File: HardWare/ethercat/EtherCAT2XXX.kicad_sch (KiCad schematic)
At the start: 5 parts, among them J1 Conn_01x02

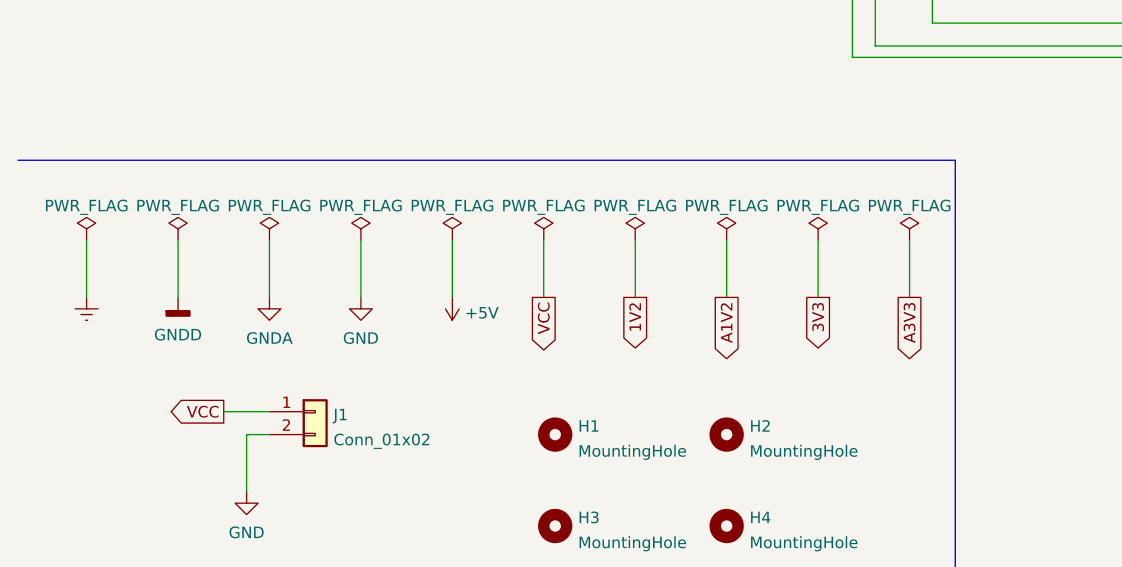
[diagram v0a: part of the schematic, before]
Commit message: Add test version
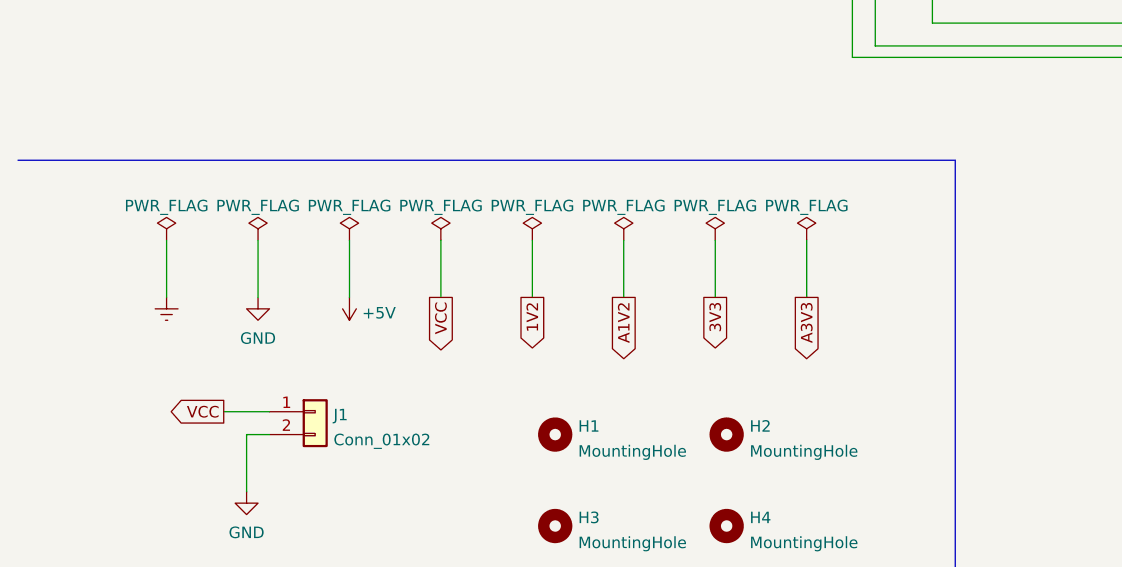
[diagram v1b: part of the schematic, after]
